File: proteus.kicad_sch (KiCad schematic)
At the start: 69 parts, among them J1 Conn_01x01, J13 Conn_01x03, J15 Sicma_56, J2 Conn_01x01, J3 Conn_01x01, J4 Conn_01x03, J5 Conn_01x05, J6 Conn_02x04_Counter_Clockwise, J9 Conn_01x04

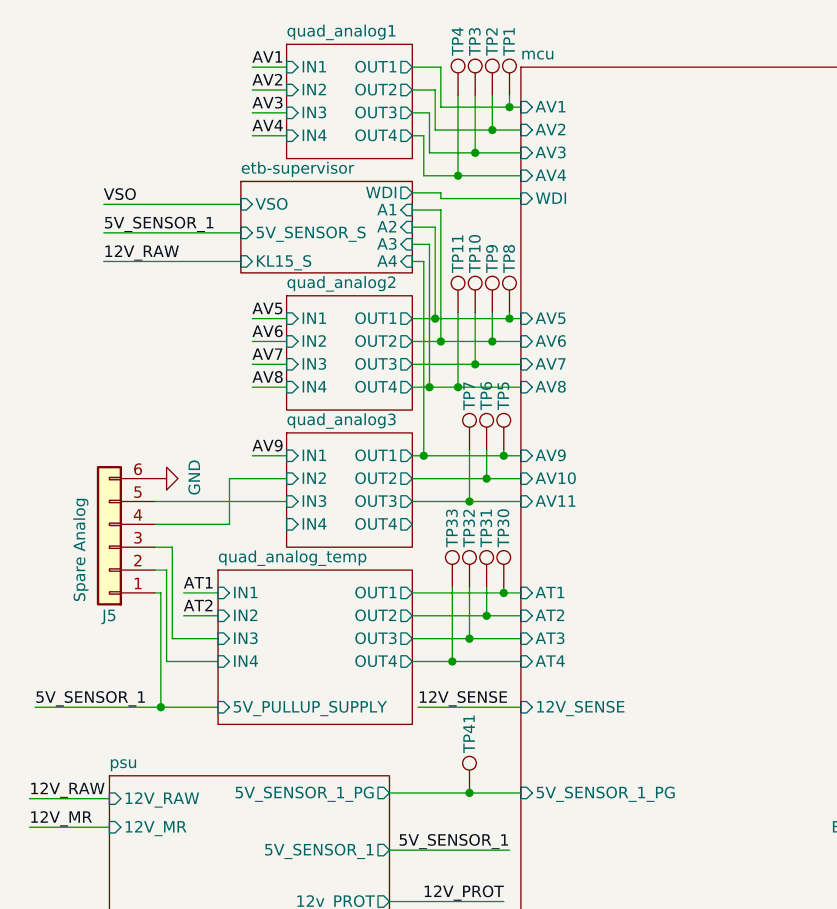
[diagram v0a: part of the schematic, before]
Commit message: Optimize
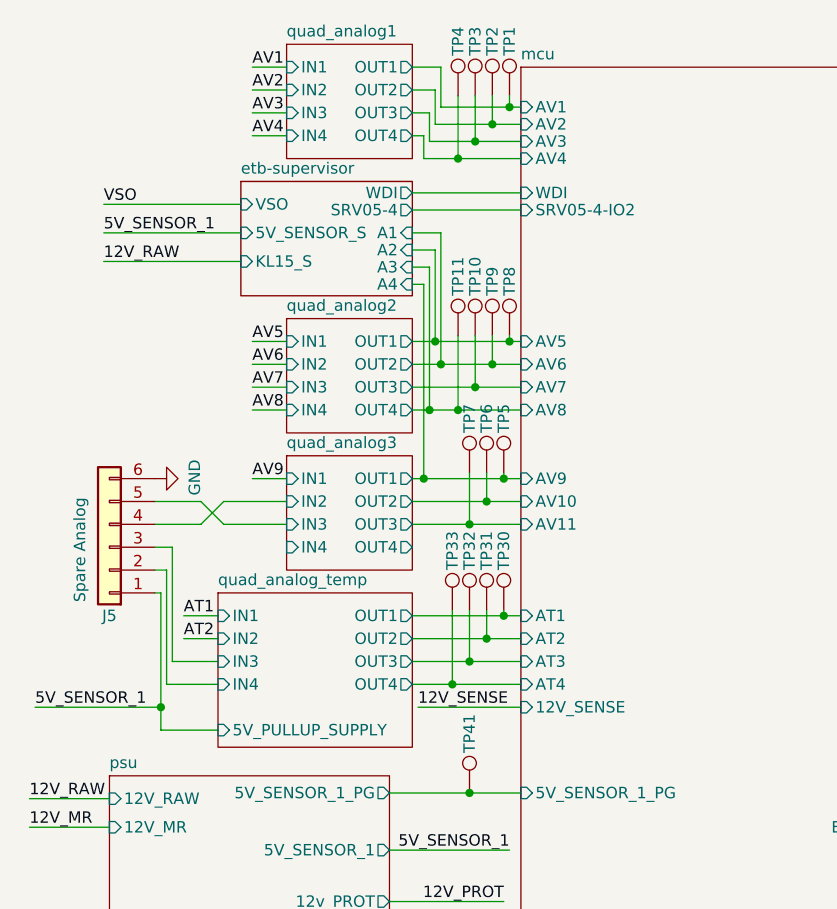
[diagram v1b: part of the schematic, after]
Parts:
- R25, R4: LCSC C106235 -> C11702
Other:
- sheet etb-supervisor ports: added SRV05-4; removed none
- sheet mcu ports: added SRV05-4-IO2; removed none
- moved on the sheet: TP10, TP11, TP30, TP31, TP32, TP33, TP5, TP6, TP7, TP8, TP9
